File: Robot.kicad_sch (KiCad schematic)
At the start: 14 parts, among them J1 XT60 4Port PDB, J2 LM2596 Buck Converter, J3 WAGO 221 - 5 Port, J4 Elegoo Mega 2560 R3, J5 Orange Pi 5, J6 Oak D Lite Camera, J7 LiDAR Sensor, U1 Cytron MDD10A, U2 Cytron MDD10A

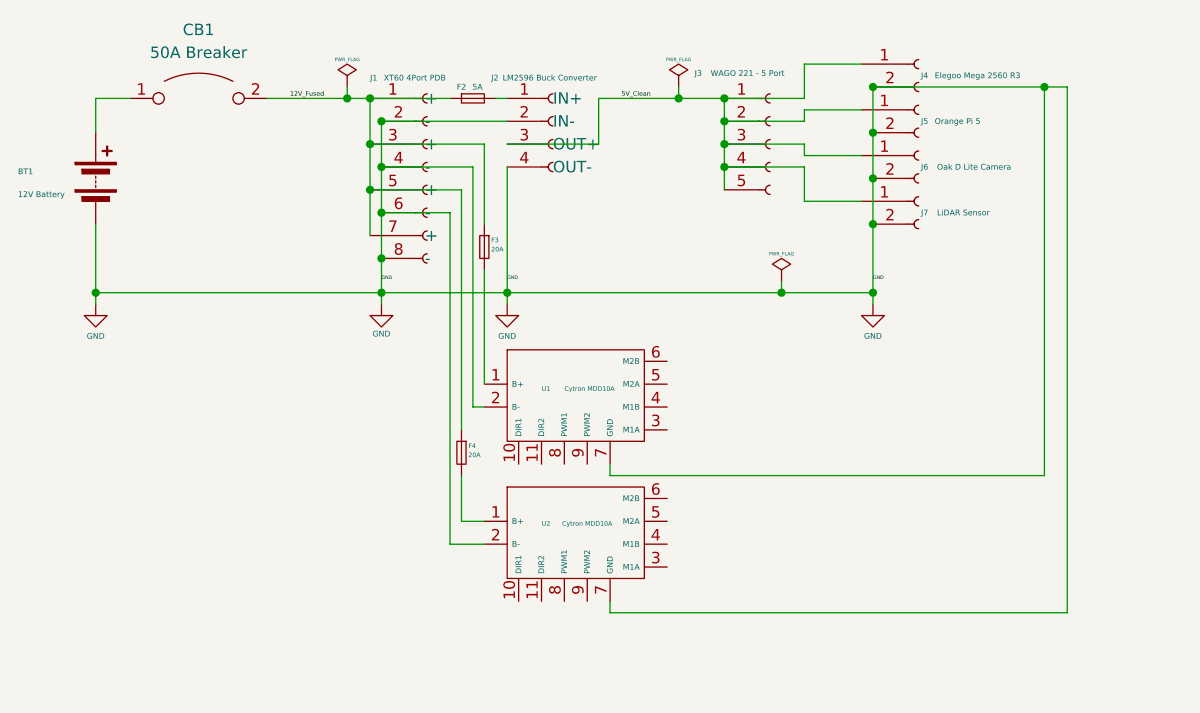
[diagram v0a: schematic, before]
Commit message: edit
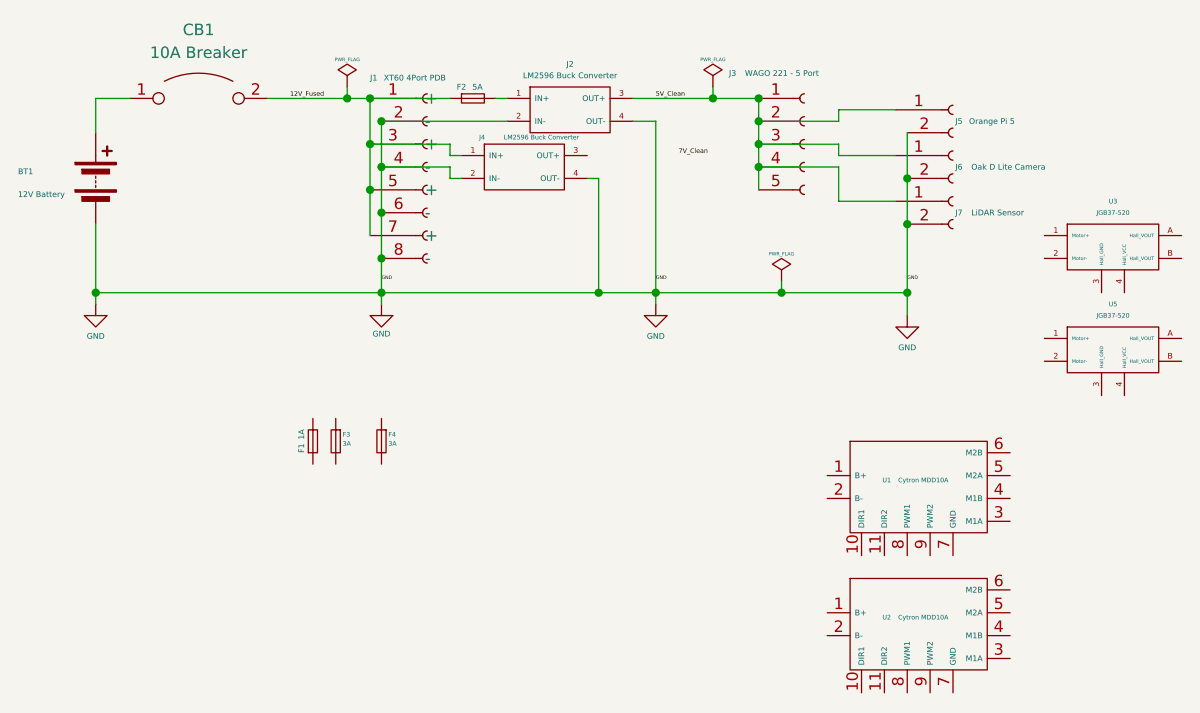
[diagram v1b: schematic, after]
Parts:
- removed J2: LM2596 Buck Converter, symbol Connector:Conn_01x04_Socket
- removed J4: Elegoo Mega 2560 R3, symbol Connector:Conn_01x02_Socket
- added F1: 1A, symbol Device:Fuse_Small
- added J2, J4: LM2596 Buck Converter, symbol Custom_Components:LM2596_Buck_Converter
- added U3, U5: JGB37-520, symbol Custom_Components:JGB37-520_12V
- CB1: value 50A Breaker -> 10A Breaker
- F3, F4: value 20A -> 3A
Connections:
- net 12V_Fused: now also J4.1 (IN+); no longer F3.1, F4.1
- net 5V_Clean: now also J2.3 (OUT+)
- net GND: now also J2.2 (IN-), J2.4 (OUT-), J4.2 (IN-), J4.4 (OUT-); no longer U1.2 (B-), U1.7 (GND), U2.2 (B-), U2.7 (GND)
- net at F2.2: now also J2.1 (IN+)
- net at F4.2: no longer U2.1 (B+)
- net at U1.1 (B+): no longer F3.2
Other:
- moved on the sheet: F3, F4, J3, J5, J6, J7
